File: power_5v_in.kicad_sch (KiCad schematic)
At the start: 16 parts, among them U19 SY6280AAC, U3 LD1117V33

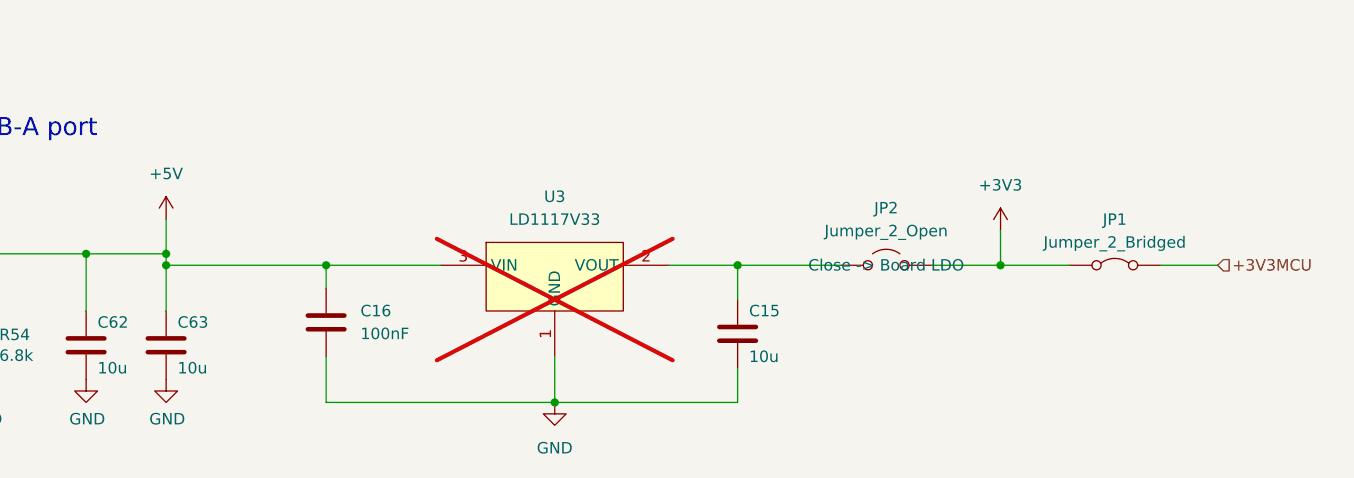
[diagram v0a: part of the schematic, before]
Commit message: WIP: Routed version, for first feedback round
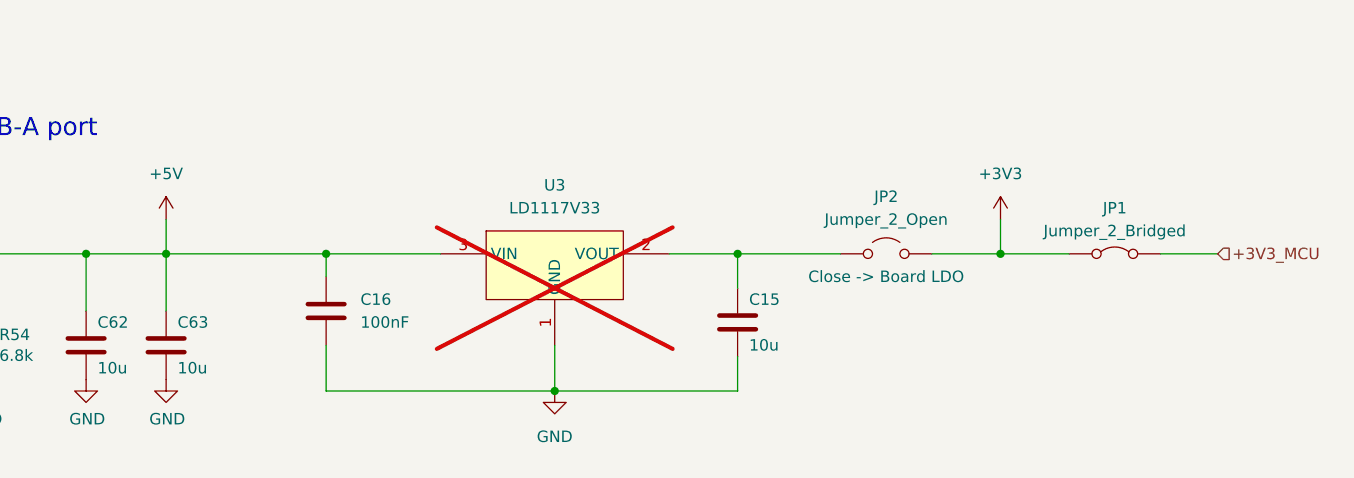
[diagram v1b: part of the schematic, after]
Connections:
- net +3V3MCU renamed +3V3_MCU
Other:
- moved on the sheet: C15, C16, JP1, JP2, U3
